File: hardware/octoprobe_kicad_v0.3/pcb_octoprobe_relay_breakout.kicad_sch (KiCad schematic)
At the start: 2 parts, among them J1001 Conn_01x20, J1002 Conn_01x20

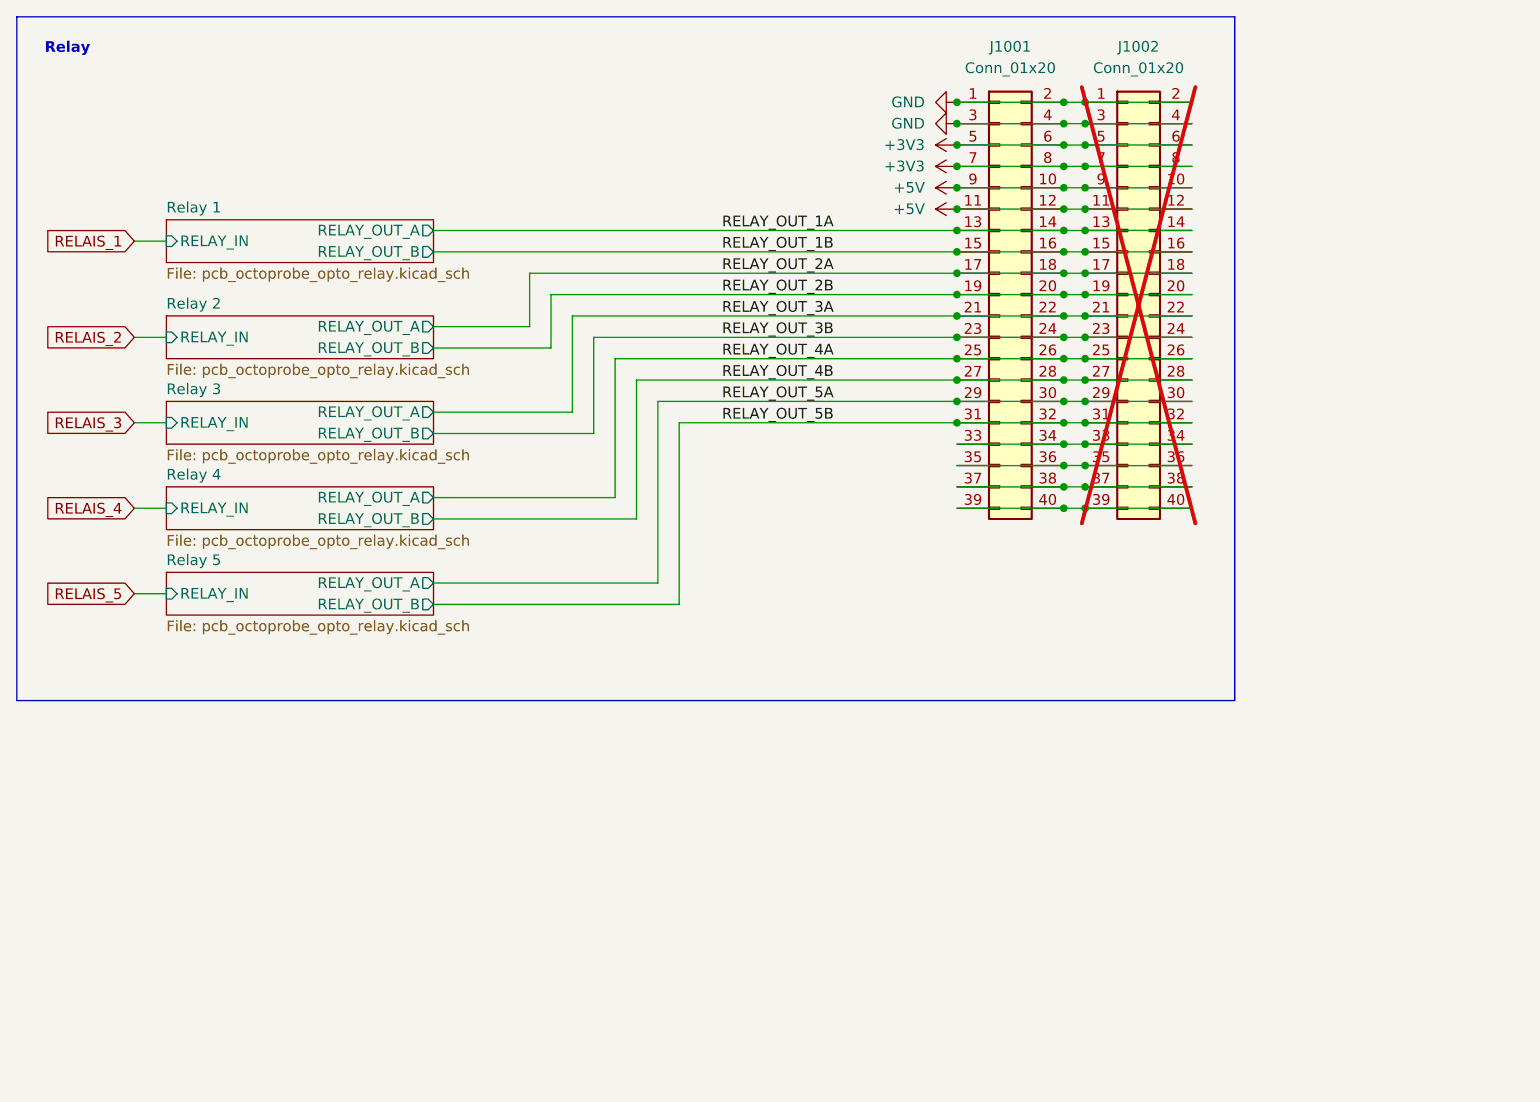
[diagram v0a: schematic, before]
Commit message: PCB: Octobus
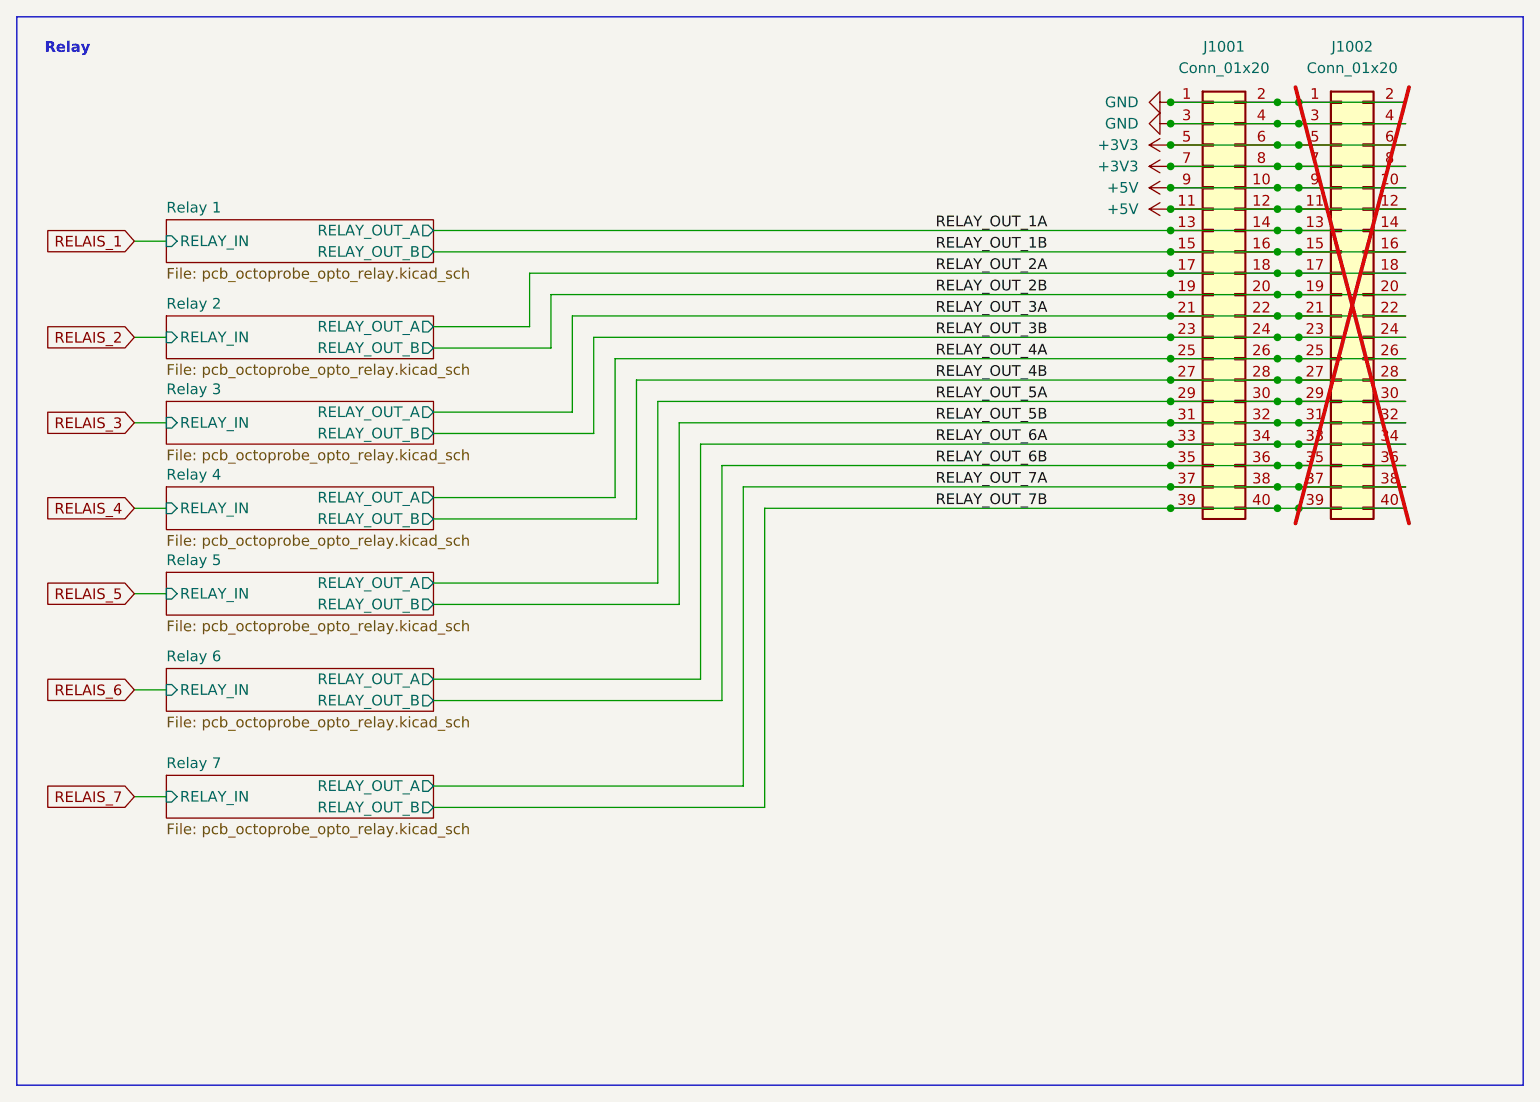
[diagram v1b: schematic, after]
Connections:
- net RELAY_OUT_6A: now reaches J1001.33 (Pin_33), J1001.34 (Pin_34), J1002.33 (Pin_33), J1002.34 (Pin_34)
- net RELAY_OUT_6B: now reaches J1001.35 (Pin_35), J1001.36 (Pin_36), J1002.35 (Pin_35), J1002.36 (Pin_36)
- net RELAY_OUT_7A: now reaches J1001.37 (Pin_37), J1001.38 (Pin_38), J1002.37 (Pin_37), J1002.38 (Pin_38)
- net RELAY_OUT_7B: now reaches J1001.39 (Pin_39), J1001.40 (Pin_40), J1002.39 (Pin_39), J1002.40 (Pin_40)
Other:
- added sheet Relay 6 (pcb_octoprobe_opto_relay.kicad_sch)
- added sheet Relay 7 (pcb_octoprobe_opto_relay.kicad_sch)
- moved on the sheet: J1001, J1002
